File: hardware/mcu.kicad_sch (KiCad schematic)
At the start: 59 parts, among them J1 TYPE-C 16PIN 2MD(073), J2 Conn_ARM_JTAG_SWD_10, J22 Conn_01x16, J3 Conn_02x03_Odd_Even, J4 Conn_02x04_Odd_Even, Q1 DMP1045U-7, Q4 SS8050, SW1 MK-12C01-G1.5, SW2 TS-1095PS-A1B2-C3D2, SW3 TS-1095PS-A1B2-C3D2, SW4 K1-1507SA-03, U1 TPS63031DSK, U10 PY25Q128HA, U2 RP2350A-QFN60, U7 24CS02, Y1 12Mhz

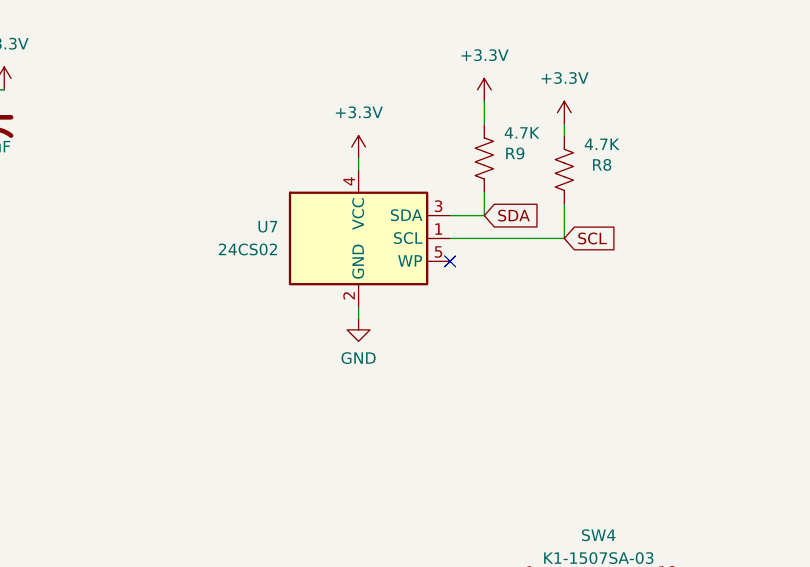
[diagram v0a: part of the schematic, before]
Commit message: Progress on station communications
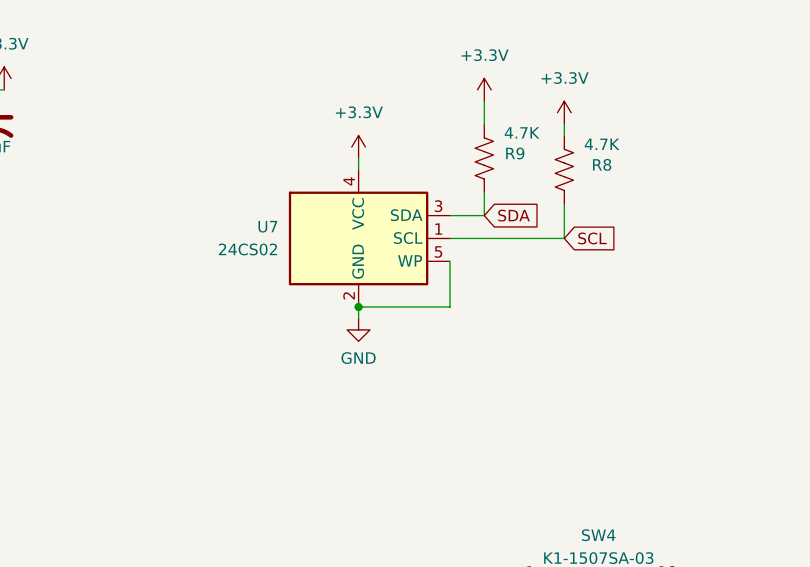
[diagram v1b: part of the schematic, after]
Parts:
- J22: footprint easyeda2kicad:CONN-SMD_16P-P0.50_5034801600_1 -> easyeda2kicad:FPC-SMD_16P-P0.50_KH-FPC0.5-H1.0SMT-16P; LCSC Part C2856801 -> C3250117
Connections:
- net GND: now also U7.5 (WP)
- no-connect marks 16 -> 15
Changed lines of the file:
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@@
 	)
 	(junction
+		(at 233.68 58.42)
+		(diameter 0)
+		(color 0 0 0 0)
+	)
+	(junction
 		(at 134.62 87.63)
 		(diameter 0)
@@
 	)
 	(no_connect
-		(at 243.84 53.34)
-	)
-	(no_connect
 		(at 199.39 130.81)
 	)
@@
 	(wire
 		(pts
+			(xy 243.84 58.42) (xy 233.68 58.42)
+		)
+		(stroke
+			(width 0)
+			(type default)
+		)
+	)
+	(wire
+		(pts
 			(xy 49.53 88.9) (xy 64.77 88.9)
 		)
@@
 	(wire
 		(pts
+			(xy 243.84 53.34) (xy 243.84 58.42)
+		)
+		(stroke
+			(width 0)
+			(type default)
+		)
+	)
+	(wire
+		(pts
 			(xy 87.63 142.24) (xy 87.63 146.05)
 		)
@@
 			)
 		)
-		(property "Footprint" "easyeda2kicad:CONN-SMD_16P-P0.50_5034801600_1"
+		(property "Footprint" "easyeda2kicad:FPC-SMD_16P-P0.50_KH-FPC0.5-H1.0SMT-16P"
 			(at 270.51 138.43 0)
 			(hide yes)
@@
 			)
 		)
-		(property "LCSC Part" "C2856801"
+		(property "LCSC Part" "C3250117"
 			(at 270.51 138.43 0)
 			(hide yes)
